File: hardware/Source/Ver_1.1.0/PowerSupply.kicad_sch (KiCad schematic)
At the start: 0 parts

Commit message: update folder hardware
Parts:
- added C29: 330uF/50V, Capacitor_SMD:CP_Elec_10x10.5, symbol automative_hexapod:Cap_Polarized_SMD_330uF_50V
- added C38: 220uF/50V, Capacitor_SMD:CP_Elec_10x10.5, symbol automative_hexapod:Cap_Polarized_SMD_220uF_50V
- added C45, C46: 1uF/16V, automative_hexapod:Ceramic_Cap_0805, symbol automative_hexapod:Ceramic_Cap_0805_1uF_16V
- added D2: MBR20100CT, automative_hexapod:TO-220-3, symbol automative_hexapod:MBR20100CT
- added L1: 27uH 5.7A, automative_hexapod:IND_CDRH127_LDNP-470MC_SUM, symbol automative_hexapod:CDRH127_1280-270_ 27uH-5.7A
- added R13: 10.5K/1%/1/8W, automative_hexapod:Res_0805, symbol automative_hexapod:Res_10.5K_0805_1%
- added R14: 2K/1%/1/8W, automative_hexapod:Res_0805, symbol automative_hexapod:Res_2K_0805_1%
- added U2: XL4005E1, automative_hexapod:TO-263-5, symbol automative_hexapod:XL4005E1
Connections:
- new net: D2.2, L1.1, U2.3 (SW)
- new net: R13.1, R14.2, U2.2 (FB)
- new net +5V: C29.1, C46.2, L1.2, R13.2
- new net GND: C29.2, C38.2, C45.1, C46.1, D2.1, R14.1, U2.1 (GND)
- new net VCC: C38.1, C45.2, U2.4 (EN), U2.5 (VIN)
- no-connect marks 0 -> 1

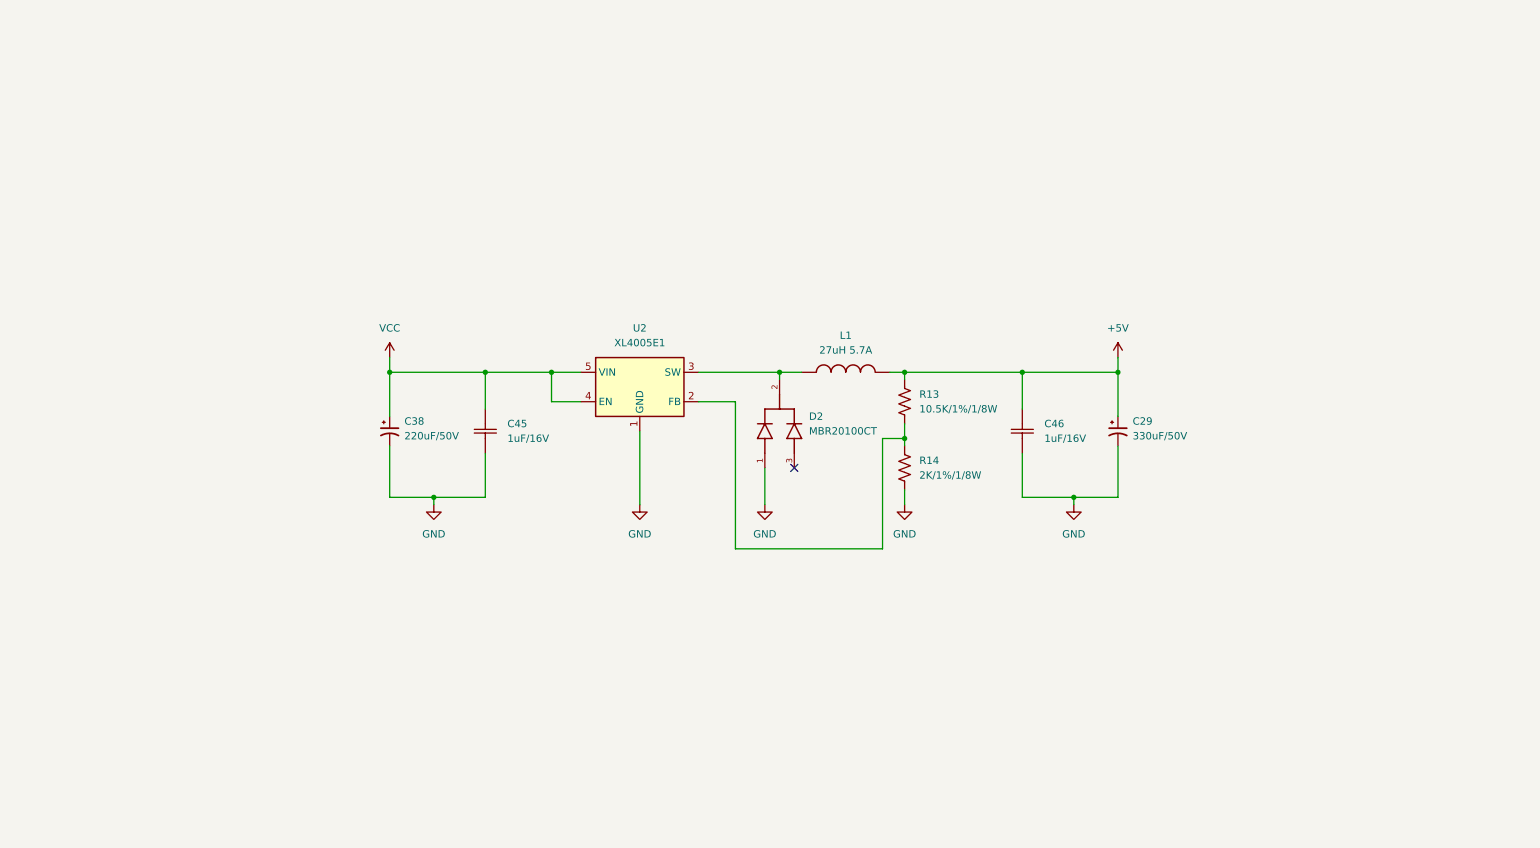
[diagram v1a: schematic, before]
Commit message: update pcb v1.1.0
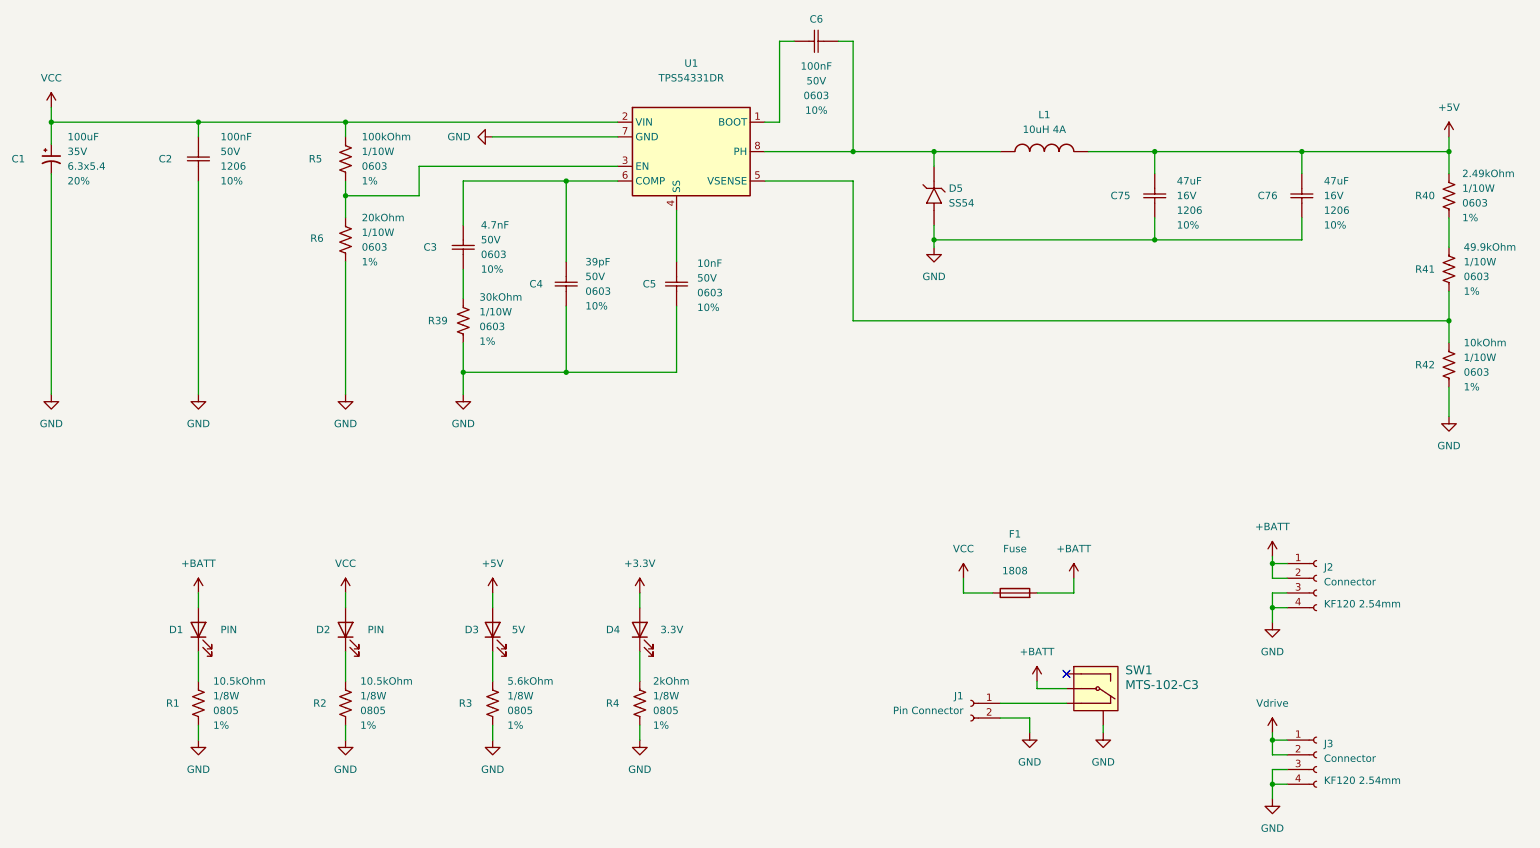
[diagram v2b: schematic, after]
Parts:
- removed C29: 330uF/50V, Capacitor_SMD:CP_Elec_10x10.5, symbol automative_hexapod:Cap_Polarized_SMD_330uF_50V
- removed C38: 220uF/50V, Capacitor_SMD:CP_Elec_10x10.5, symbol automative_hexapod:Cap_Polarized_SMD_220uF_50V
- removed C45, C46: 1uF/16V, automative_hexapod:Ceramic_Cap_0805, symbol automative_hexapod:Ceramic_Cap_0805_1uF_16V
- removed D2: MBR20100CT, automative_hexapod:TO-220-3, symbol automative_hexapod:MBR20100CT
- removed L1: 27uH 5.7A, automative_hexapod:IND_CDRH127_LDNP-470MC_SUM, symbol automative_hexapod:CDRH127_1280-270_ 27uH-5.7A
- removed R13: 10.5K/1%/1/8W, automative_hexapod:Res_0805, symbol automative_hexapod:Res_10.5K_0805_1%
- removed R14: 2K/1%/1/8W, automative_hexapod:Res_0805, symbol automative_hexapod:Res_2K_0805_1%
- removed U2: XL4005E1, automative_hexapod:TO-263-5, symbol automative_hexapod:XL4005E1
- added C1: 100uF, automative_hexapod:CP_Elec_6.3x5.4, symbol automative_hexapod:Cap_Polarized_SMD_100uF_35V
- added C2: 100nF, automative_hexapod:Ceramic_Cap_1206, symbol automative_hexapod:Ceramic_Cap_1206_100nF_50V
- added C3: 4.7nF, automative_hexapod:Ceramic_Cap_0603, symbol automative_hexapod:Ceramic_Cap_0603_4.7nF_50V
- added C4: 39pF, automative_hexapod:Ceramic_Cap_0603, symbol automative_hexapod:Ceramic_Cap_0603_39pF_50V
- added C5: 10nF, automative_hexapod:Ceramic_Cap_0603, symbol automative_hexapod:Ceramic_Cap_0603_10nF_50V
- added C6: 100nF, automative_hexapod:Ceramic_Cap_0603, symbol automative_hexapod:Ceramic_Cap_0603_100nF_50V
- added C75, C76: 47uF, automative_hexapod:Ceramic_Cap_1206, symbol automative_hexapod:Ceramic_Cap_1206_47uF_16V
- added D1, D2: PIN, automative_hexapod:LED_0805, symbol automative_hexapod:LED_0805
- added D3: 5V, automative_hexapod:LED_0805, symbol automative_hexapod:LED_0805
- added D4: 3.3V, automative_hexapod:LED_0805, symbol automative_hexapod:LED_0805
- added D5: SS54, automative_hexapod:D_SMA, symbol automative_hexapod:SS54
- added F1: Fuse, automative_hexapod:FUSE_SMD_1808, symbol automative_hexapod:Fuse_1808
- added J1: Pin Connector, automative_hexapod:Connector-Pin, symbol automative_hexapod:Pin Connector
- added J2, J3: Connector, automative_hexapod:TerminalBlock_Phoenix_MKDS-1,5-4-5.08_1x04_P5.08mm_Horizontal, symbol automative_hexapod:KF120-4-V Domino
- added L1: 10uH 4A, automative_hexapod:Inductor_0630, symbol automative_hexapod:0630_10uH-4A
- added R1, R2: 10.5kOhm, automative_hexapod:Res_0805, symbol automative_hexapod:Res_10.5K_0805_1%
- added R3: 5.6kOhm, automative_hexapod:Res_0805, symbol automative_hexapod:Res_5.6K_0805_1%
- added R39: 30kOhm, automative_hexapod:Res_0603, symbol automative_hexapod:Res_30K_0603_1%
- added R4: 2kOhm, automative_hexapod:Res_0805, symbol automative_hexapod:Res_2K_0805_1%
- added R40: 2.49kOhm, automative_hexapod:Res_0603, symbol automative_hexapod:Res_2.49K_0603_1%
- added R41: 49.9kOhm, automative_hexapod:Res_0603, symbol automative_hexapod:Res_49.9K_0603_1%
- added R42: 10kOhm, automative_hexapod:Res_0603, symbol automative_hexapod:Res_10K_0603_1%
- added R5: 100kOhm, automative_hexapod:Res_0603, symbol automative_hexapod:Res_100K_0603_1%
- added R6: 20kOhm, automative_hexapod:Res_0603, symbol automative_hexapod:Res_20K_0603_1%
- added SW1: MTS-102-C3, automative_hexapod:MTS-102-C3, symbol automative_hexapod:MTS-102-C3
- added U1: TPS54331DR, automative_hexapod:SOIC-8, symbol automative_hexapod:TPS54331DR
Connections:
- net +5V: now also C75.2, C76.2, D3.2 (A), L1.2, R40.2
- net GND: now also C1.2, C2.2, C4.1, C5.1, C75.1, C76.1, D5.1 (A), J1.2 (Pin_2), J2.3 (Pin_3), J2.4 (Pin_4), J3.3 (Pin_3), J3.4 (Pin_4), R1.1, R2.1, R3.1, R39.1, R4.1, R42.1, R6.1, SW1.SH, U1.7 (GND)
- net VCC: now also C1.1, C2.1, D2.2 (A), F1.1, R5.2, U1.2 (VIN)
- new net: D4.1 (K), R4.2
- new net: D1.1 (K), R1.2
- new net: C6.2, D5.2 (K), L1.1, U1.8 (PH)
- new net: D3.1 (K), R3.2
- new net: R41.1, R42.2, U1.5 (VSENSE)
- new net: R40.1, R41.2
- new net: J1.1 (Pin_1), SW1.1
- new net: R5.1, R6.2, U1.3 (EN)
- new net: C6.1, U1.1 (BOOT)
- new net: C5.2, U1.4 (SS)
- new net: C3.2, C4.2, U1.6 (COMP)
- new net: D2.1 (K), R2.2
- new net: C3.1, R39.2
- new net +3.3V: D4.2 (A)
- new net +BATT: D1.2 (A), F1.2, J2.1 (Pin_1), J2.2 (Pin_2), SW1.2
- new net Vdrive: J3.1 (Pin_1), J3.2 (Pin_2)
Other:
- title: (none) -> Power Supply
